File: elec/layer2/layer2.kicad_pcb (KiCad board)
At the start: 2 copper layers, 1 part

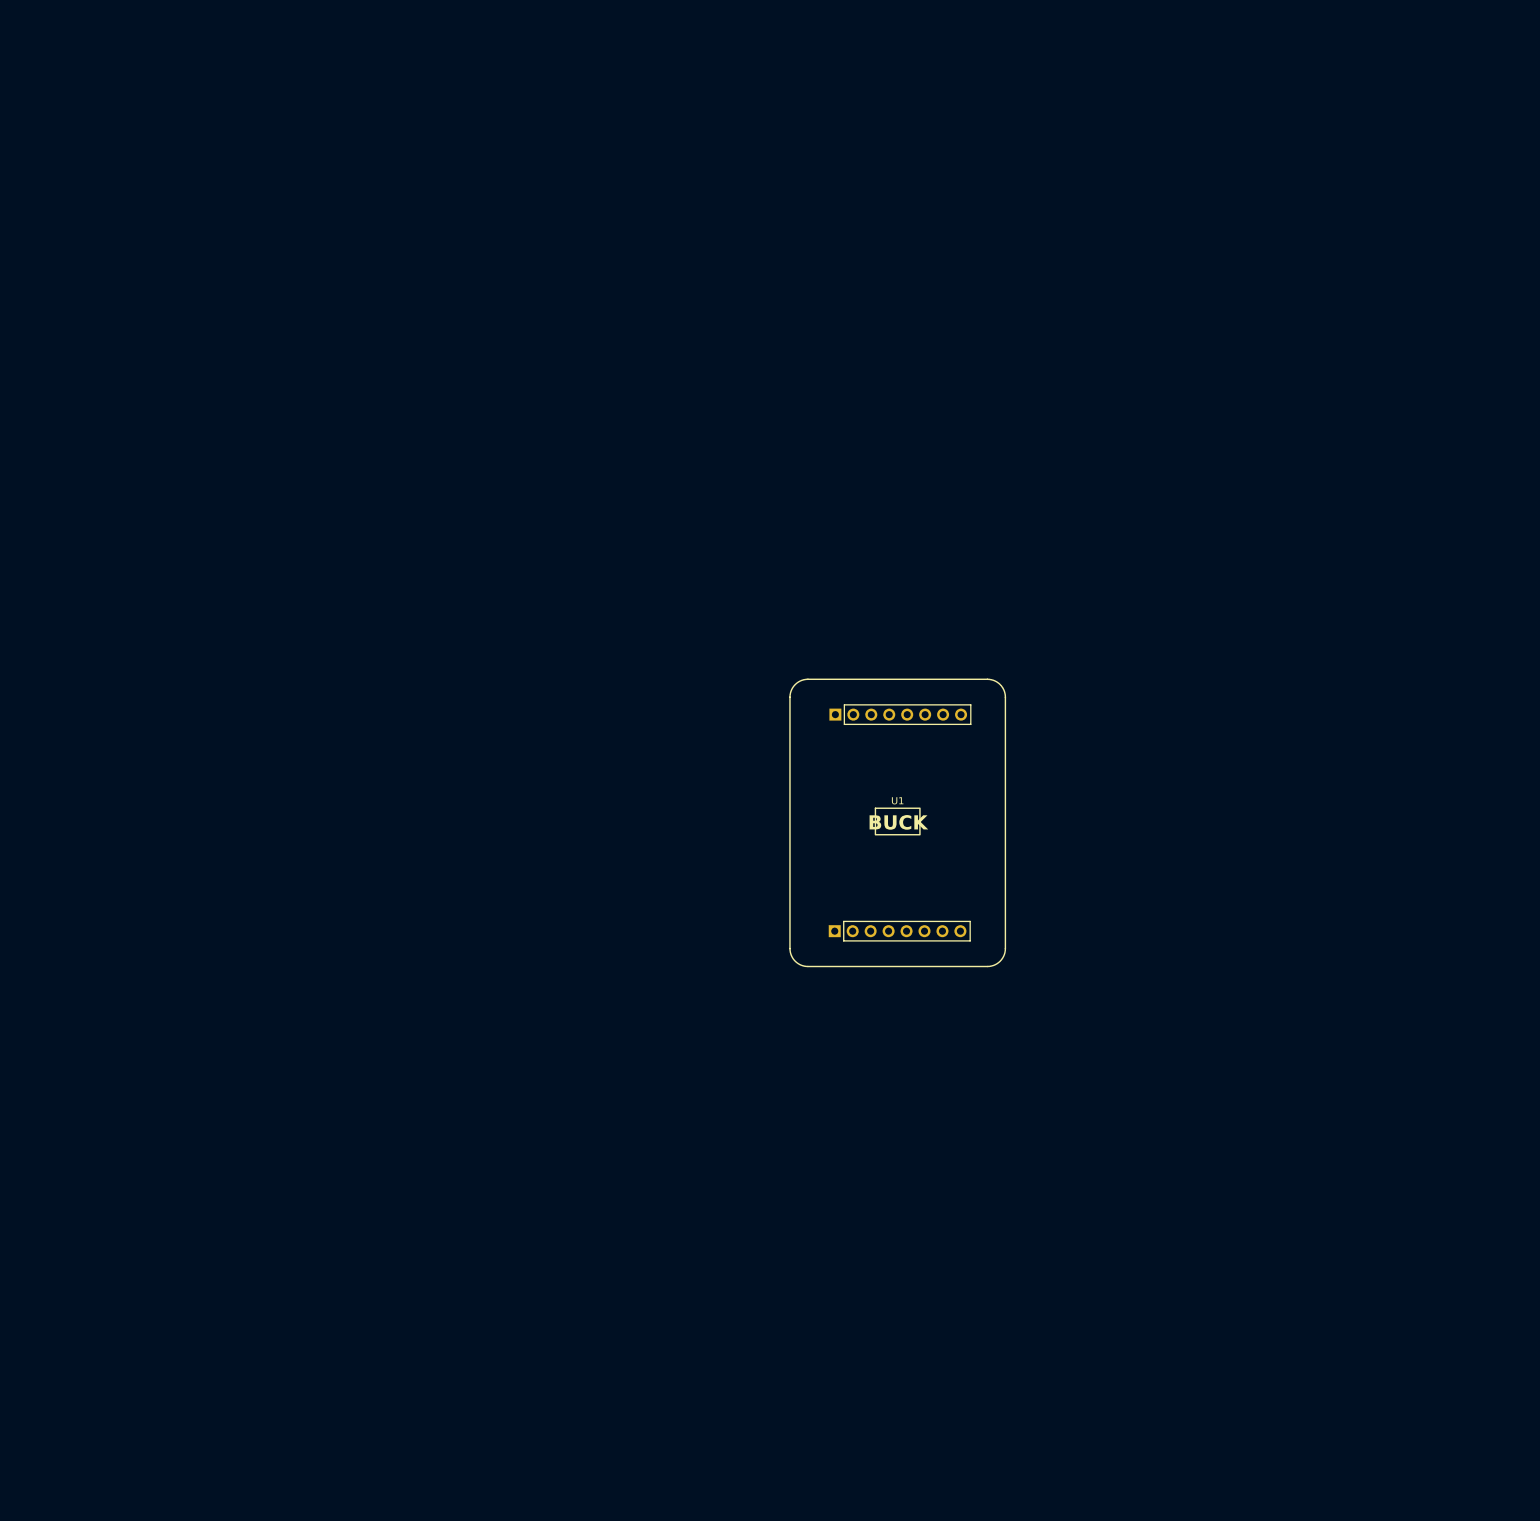
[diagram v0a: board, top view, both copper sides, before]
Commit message: feat: did something
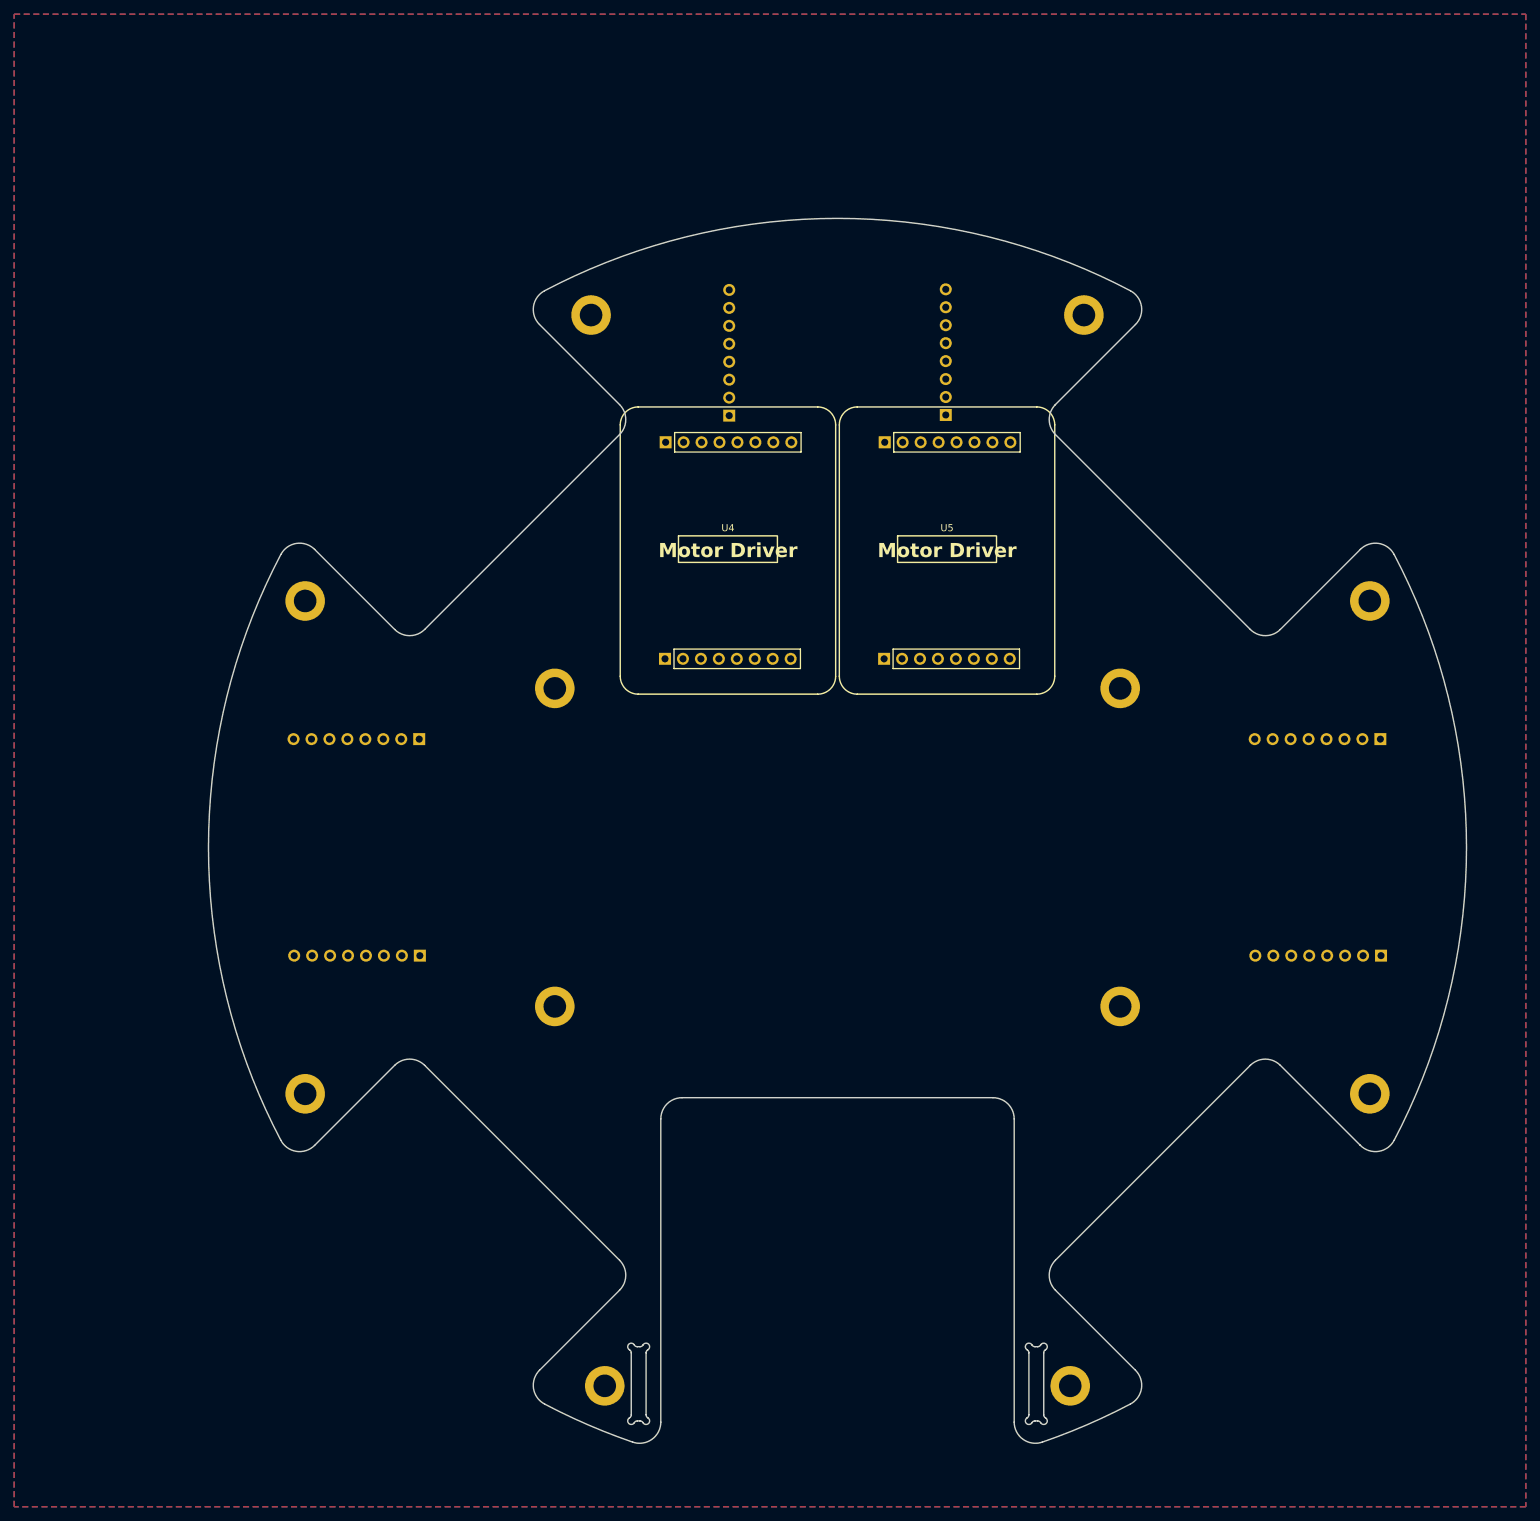
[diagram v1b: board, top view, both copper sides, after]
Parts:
- added H1: MountingHole, MountingHole:MountingHole_3.2mm_M3_DIN965_Pad, F.Cu at (80.9, 33.9)
- added H10: MountingHole, MountingHole:MountingHole_3.2mm_M3_DIN965_Pad, F.Cu at (191.1, 144.1)
- added H11: MountingHole, MountingHole:MountingHole_3.2mm_M3_DIN965_Pad, F.Cu at (82.9, 185.4)
- added H12: MountingHole, MountingHole:MountingHole_3.2mm_M3_DIN965_Pad, F.Cu at (148.7, 185.4)
- added H2: MountingHole, MountingHole:MountingHole_3.2mm_M3_DIN965_Pad, F.Cu at (150.7, 33.9)
- added H3: MountingHole, MountingHole:MountingHole_3.2mm_M3_DIN965_Pad, F.Cu at (40.5, 74.4)
- added H4: MountingHole, MountingHole:MountingHole_3.2mm_M3_DIN965_Pad, F.Cu at (191.1, 74.4)
- added H5: MountingHole, MountingHole:MountingHole_3.2mm_M3_DIN965_Pad, F.Cu at (75.8, 86.7)
- added H6: MountingHole, MountingHole:MountingHole_3.2mm_M3_DIN965_Pad, F.Cu at (155.8, 86.7)
- added H7: MountingHole, MountingHole:MountingHole_3.2mm_M3_DIN965_Pad, F.Cu at (75.8, 131.7)
- added H8: MountingHole, MountingHole:MountingHole_3.2mm_M3_DIN965_Pad, F.Cu at (155.8, 131.7)
- added H9: MountingHole, MountingHole:MountingHole_3.2mm_M3_DIN965_Pad, F.Cu at (40.5, 144.1)
- added U2: ~, layer2-pcb-footprints:motor-driver-module, B.Cu at (47.8, 109.2)
- added U3: ~, layer2-pcb-footprints:motor-driver-module, B.Cu at (183.8, 109.2)
- added U4: ~, layer2-pcb-footprints:motor-driver-module, F.Cu at (100.3, 67.2)
- added U5: ~, layer2-pcb-footprints:motor-driver-module, F.Cu at (131.3, 67.2)
- U1: moved to B.Cu
- moved U1 67.1 mm to (115.8, 39.2), turned to 90 degrees
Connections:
- U1 pad 2: unconnected-(U1-GND-Pad2) -> GND
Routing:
- added copper zone on B.Cu, net GND
- added copper zone on F.Cu, net GND
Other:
- board outline added: 178 x 173.3 mm
